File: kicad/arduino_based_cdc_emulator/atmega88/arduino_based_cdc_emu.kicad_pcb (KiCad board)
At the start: 2 copper layers, 25.4 x 23.2 mm, 14 parts, among them IC1 ATMEGA88-A, P1 CONN_1, P2 CONN_2, P3 CONN_3, U1 78L05, X1 20MHz

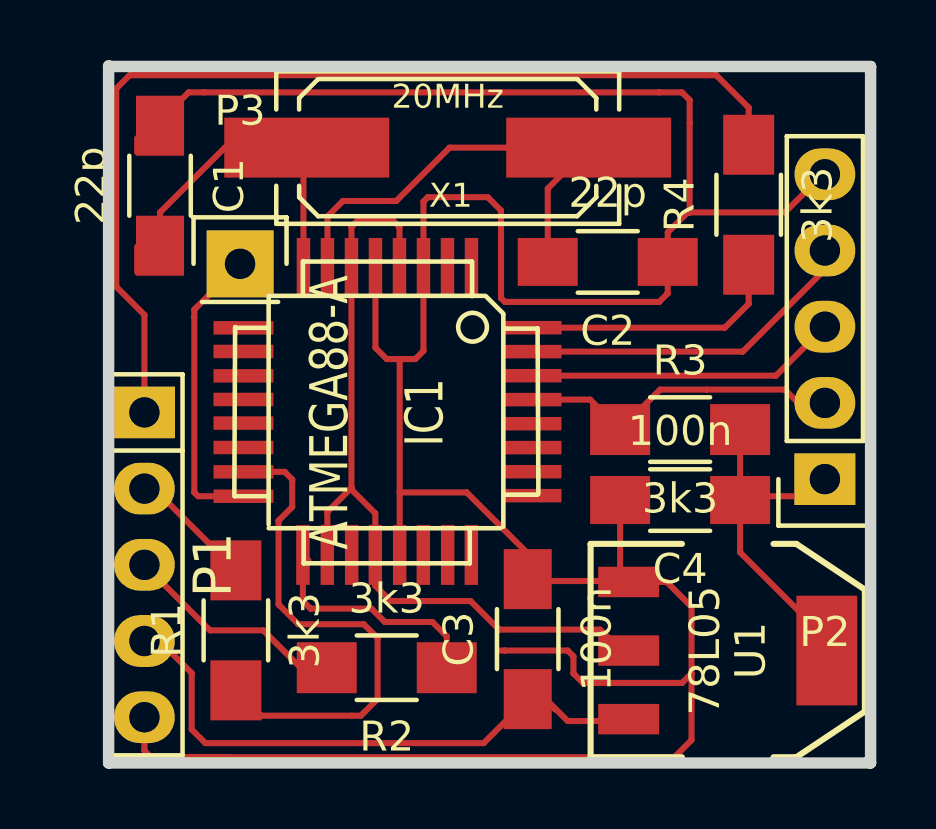
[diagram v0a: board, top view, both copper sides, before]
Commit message: updates
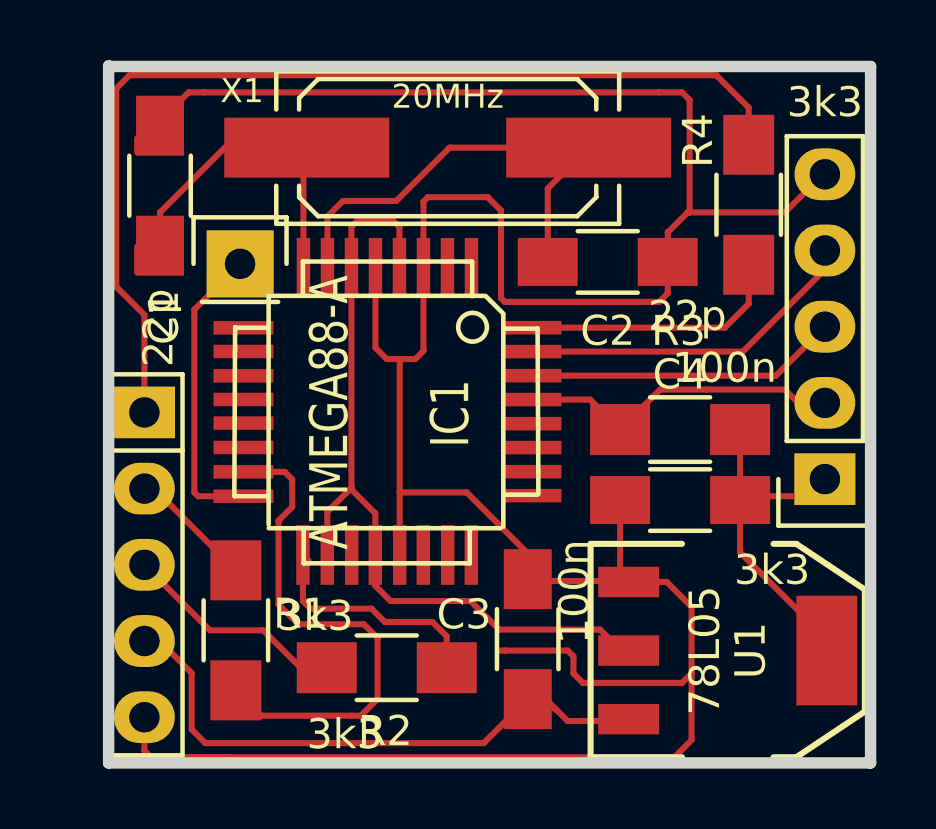
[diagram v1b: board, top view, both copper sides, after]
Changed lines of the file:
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@@
-(kicad_pcb (version 4) (host pcbnew 0.201511171411+6319~30~ubuntu14.04.1-product)
+(kicad_pcb (version 20160815) (host pcbnew 4.1.0-alpha+201608211231+7083~46~ubuntu16.04.1-product)
   (general
     (links 34)
     (no_connects 1)
-    (area 98.4385 95.5548 137.922002 124.015501)
+    (area 99.797799 95.8088 137.922001 123.88946)
     (thickness 1.6002)
     (drawings 6)
@@
     (pad_to_mask_clearance 0.254)
     (aux_axis_origin 0 0)
-    (visible_elements FFFFFF7F)
+    (visible_elements FFFEFF7F)
     (pcbplotparams
       (layerselection 0x00030_80000001)
@@
       (hpglpenspeed 20)
       (hpglpendiameter 15)
-      (hpglpenoverlay 2)
       (psnegative false)
       (psa4output false)
@@
     (uvia_dia 0.508)
     (uvia_drill 0.127)
+    (diff_pair_gap 0.25)
+    (diff_pair_width 0.2)
     (add_net +12V)
     (add_net +5V)
@@
     (tags "capacitor 1206")
     (attr smd)
-    (fp_text reference C1 (at 0 -2.3 270) (layer F.SilkS)
-      (effects (font (size 1 1) (thickness 0.15)))
-    )
-    (fp_text value 22p (at 0 2.3 270) (layer F.SilkS)
+    (fp_text reference C1 (at 4.3925 -0.1325 270) (layer F.SilkS)
+      (effects (font (size 1 1) (thickness 0.15)))
+    )
+    (fp_text value 22p (at 4.7371 0.0508 270) (layer F.SilkS)
       (effects (font (size 1 1) (thickness 0.15)))
     )
@@
       (effects (font (size 1 1) (thickness 0.15)))
     )
-    (fp_text value 22p (at 0 2.3 180) (layer F.SilkS)
+    (fp_text value 22p (at -2.6543 -1.8034 180) (layer F.SilkS)
       (effects (font (size 1 1) (thickness 0.15)))
     )
@@
     (tags "capacitor 1206")
     (attr smd)
-    (fp_text reference C3 (at 0 -2.3 90) (layer F.SilkS)
-      (effects (font (size 1 1) (thickness 0.15)))
-    )
-    (fp_text value 100n (at 0 2.3 90) (layer F.SilkS)
+    (fp_text reference C3 (at 0.8205 -2.123 180) (layer F.SilkS)
+      (effects (font (size 1 1) (thickness 0.15)))
+    )
+    (fp_text value 100n (at 1.57734 1.55448 90) (layer F.SilkS)
       (effects (font (size 1 1) (thickness 0.15)))
     )
@@
     (tags "capacitor 1206")
     (attr smd)
-    (fp_text reference C4 (at 0 -2.3 180) (layer F.SilkS)
-      (effects (font (size 1 1) (thickness 0.15)))
-    )
-    (fp_text value 100n (at 0 2.3 180) (layer F.SilkS)
+    (fp_text reference C4 (at 0.003 4.185 360) (layer F.SilkS)
+      (effects (font (size 1 1) (thickness 0.15)))
+    )
+    (fp_text value 100n (at -1.47828 4.40436 180) (layer F.SilkS)
       (effects (font (size 1 1) (thickness 0.15)))
     )
@@
   (module SMD_Packages:TQFP-32 (layer Front)
     (at 109.474 112.014 270)
-    (fp_text reference IC1 (at 0 -1.27 270) (layer F.SilkS)
+    (fp_text reference IC1 (at 0.036 -2.126 270) (layer F.SilkS)
       (effects (font (size 1.27 1.016) (thickness 0.2032)))
     )
@@
     (descr "Through hole pin header")
     (tags "pin header")
-    (fp_text reference P1 (at 0 -2.286 270) (layer F.SilkS)
+    (fp_text reference P1 (at 0 -2.286 270) (layer F.SilkS) hide
       (effects (font (size 1.27 1.27) (thickness 0.2032)))
     )
@@
     (tags "resistor 1206")
     (attr smd)
-    (fp_text reference R1 (at 0 -2.3 90) (layer F.SilkS)
-      (effects (font (size 1 1) (thickness 0.15)))
-    )
-    (fp_text value 3k3 (at 0 2.3 90) (layer F.SilkS)
+    (fp_text reference R1 (at 0.55118 2.15646) (layer F.SilkS)
+      (effects (font (size 1 1) (thickness 0.15)))
+    )
+    (fp_text value 3k3 (at 0.47752 2.65176 180) (layer F.SilkS)
       (effects (font (size 1 1) (thickness 0.15)))
     )
@@
     (tags "resistor 1206")
     (attr smd)
-    (fp_text reference R2 (at 0 -2.3 180) (layer F.SilkS)
-      (effects (font (size 1 1) (thickness 0.15)))
-    )
-    (fp_text value 3k3 (at 0 2.3 180) (layer F.SilkS)
+    (fp_text reference R2 (at 0.0508 -2.11328 180) (layer F.SilkS)
+      (effects (font (size 1 1) (thickness 0.15)))
+    )
+    (fp_text value 3k3 (at 1.40208 -2.21996 180) (layer F.SilkS)
       (effects (font (size 1 1) (thickness 0.15)))
     )
@@
     (tags "resistor 1206")
     (attr smd)
-    (fp_text reference R3 (at 0 -2.3) (layer F.SilkS)
-      (effects (font (size 1 1) (thickness 0.15)))
-    )
-    (fp_text value 3k3 (at 0 2.3) (layer F.SilkS)
+    (fp_text reference R3 (at -0.053 -3.2855) (layer F.SilkS)
+      (effects (font (size 1 1) (thickness 0.15)))
+    )
+    (fp_text value 3k3 (at 3.06832 4.68122) (layer F.SilkS)
       (effects (font (size 1 1) (thickness 0.15)))
     )
@@
     (tags "resistor 1206")
     (attr smd)
-    (fp_text reference R4 (at 0 -2.3 90) (layer F.SilkS)
-      (effects (font (size 1 1) (thickness 0.15)))
-    )
-    (fp_text value 3k3 (at 0 2.3 90) (layer F.SilkS)
+    (fp_text reference R4 (at 2.1425 -1.689 90) (layer F.SilkS)
+      (effects (font (size 1 1) (thickness 0.15)))
+    )
+    (fp_text value 3k3 (at 3.4163 2.54 180) (layer F.SilkS)
       (effects (font (size 1 1) (thickness 0.15)))
     )
@@
   (module Crystals_Oscillators_SMD:Q_49U3HMS (layer Front)
     (at 111.506 103.1875 180)
-    (fp_text reference X1 (at -0.1 -1.6 180) (layer F.SilkS)
+    (fp_text reference X1 (at 6.856 1.8875 180) (layer F.SilkS)
       (effects (font (size 0.8 0.8) (thickness 0.15)))
     )
@@
     (descr "Through hole pin header")
     (tags "pin header")
-    (fp_text reference P2 (at 0 -5.1 180) (layer F.SilkS)
+    (fp_text reference P2 (at 0 -5.1 180) (layer F.SilkS) hide
       (effects (font (size 1 1) (thickness 0.15)))
     )
@@
     (descr "Through hole pin header")
     (tags "pin header")
-    (fp_text reference P3 (at 0 -5.1) (layer F.SilkS)
+    (fp_text reference P3 (at 0 -5.1) (layer F.SilkS) hide
       (effects (font (size 1 1) (thickness 0.15)))
     )
@@
   (segment (start 123.444 118.872) (end 124.206 119.634) (width 0.2032) (layer Front) (net 1))
   (segment (start 121.253 116.681) (end 124.206 119.634) (width 0.2032) (layer Front) (net 1))
-  (segment (start 107.474 120.523) (end 106.6038 120.523) (width 0.2032) (layer Front) (net 2))
-  (segment (start 106.6038 120.523) (end 105.3592 119.2784) (width 0.2032) (layer Front) (net 2))
+  (segment (start 107.474 120.523) (end 106.6038 120.523) (width 0.2032) (layer Front) (net 2) (status 30))
+  (segment (start 106.6038 120.523) (end 105.3592 119.2784) (width 0.2032) (layer Front) (net 2) (status 10))
   (segment (start 105.3592 119.2784) (end 103.5812 119.2784) (width 0.2032) (layer Front) (net 2))
   (segment (start 103.5812 119.2784) (end 101.3968 117.094) (width 0.2032) (layer Front) (net 2))
-  (segment (start 106.712 120.8405) (end 106.712 120.555) (width 0.2032) (layer Front) (net 2))
+  (segment (start 106.712 120.8405) (end 106.712 120.555) (width 0.2032) (layer Front) (net 2) (status 30))
   (segment (start 101.3968 114.554) (end 101.7204 114.554) (width 0.2032) (layer Front) (net 3))
   (segment (start 101.7204 114.554) (end 104.4448 117.2784) (width 0.2032) (layer Front) (net 3))
@@
   (segment (start 114.808 121.634) (end 114.808 122.428) (width 0.2032) (layer Front) (net 8))
   (segment (start 115.094 121.92) (end 114.808 121.634) (width 0.2032) (layer Front) (net 8))
-  (segment (start 111.474 120.523) (end 111.474 119.475) (width 0.2032) (layer Front) (net 9))
+  (segment (start 111.474 120.523) (end 111.474 119.475) (width 0.2032) (layer Front) (net 9) (status 10))
   (segment (start 110.998 118.999) (end 109.4105 118.999) (width 0.2032) (layer Front) (net 9))
   (segment (start 111.474 119.475) (end 110.998 118.999) (width 0.2032) (layer Front) (net 9))
@@
   (segment (start 106.934 118.5545) (end 108.966 118.5545) (width 0.2032) (layer Front) (net 9))
   (segment (start 106.68 118.3005) (end 106.934 118.5545) (width 0.2032) (layer Front) (net 9))
-  (segment (start 111.347 120.4595) (end 110.8075 120.4595) (width 0.2032) (layer Front) (net 9))
+  (segment (start 111.347 120.4595) (end 110.8075 120.4595) (width 0.2032) (layer Front) (net 9) (status 30))
   (segment (start 106.8705 116.9543) (end 106.68 116.7638) (width 0.2032) (layer Front) (net 9))
-  (segment (start 111.347 120.4595) (end 111.1885 120.4595) (width 0.2032) (layer Front) (net 9))
+  (segment (start 111.347 120.4595) (end 111.1885 120.4595) (width 0.2032) (layer Front) (net 9) (status 30))
   (segment (start 114.3 109.18952) (end 120.74398 109.18952) (width 0.2032) (layer Front) (net 10))
   (segment (start 121.539 108.3945) (end 121.539 107.0925) (width 0.2032) (layer Front) (net 10))
